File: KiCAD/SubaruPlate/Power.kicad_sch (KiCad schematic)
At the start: 15 parts, among them J3 DF51A-2P-2DSA, U2 NCV8114BSN330T1G

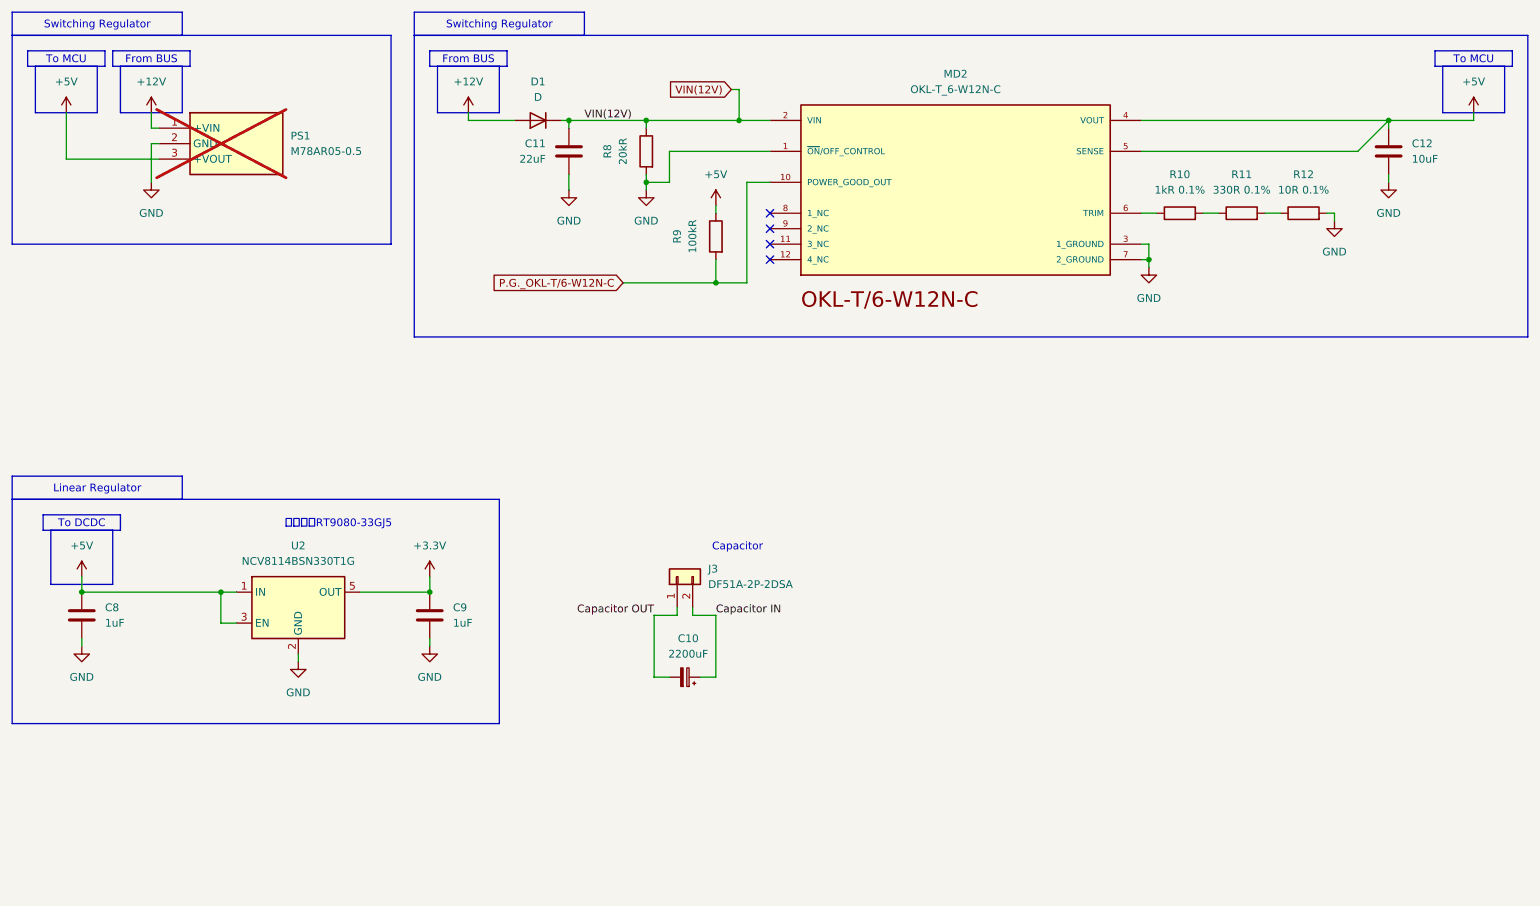
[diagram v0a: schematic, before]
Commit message: Build-2完成．発注．
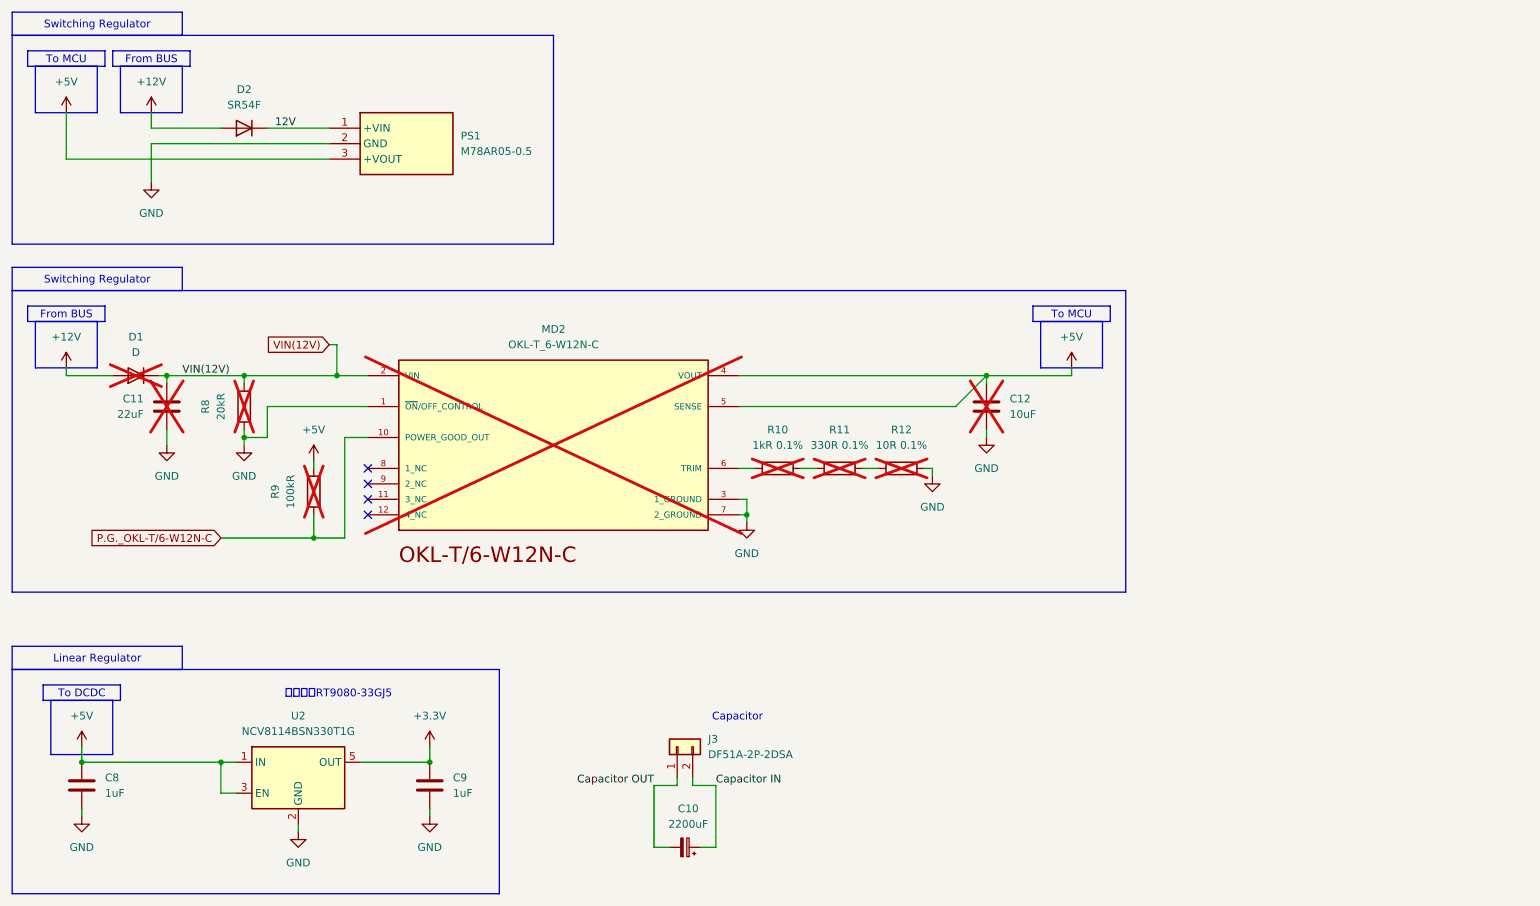
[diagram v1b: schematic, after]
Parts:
- added D2: SR54F, Diode_SMD:D_SMA, symbol Device:D
- C11, C12, D1, MD2, R10, R11, R12, R8, R9: now not fitted; now left out of the parts list
- PS1: now fitted; now in the parts list
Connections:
- net +12V: now also D2.2 (A); no longer PS1.1 (+VIN)
- new net 12V: D2.1 (K), PS1.1 (+VIN)
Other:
- moved on the sheet: C10, C8, C9, J3, U2
